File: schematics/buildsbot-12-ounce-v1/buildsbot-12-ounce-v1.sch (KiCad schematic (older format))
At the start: 15 parts

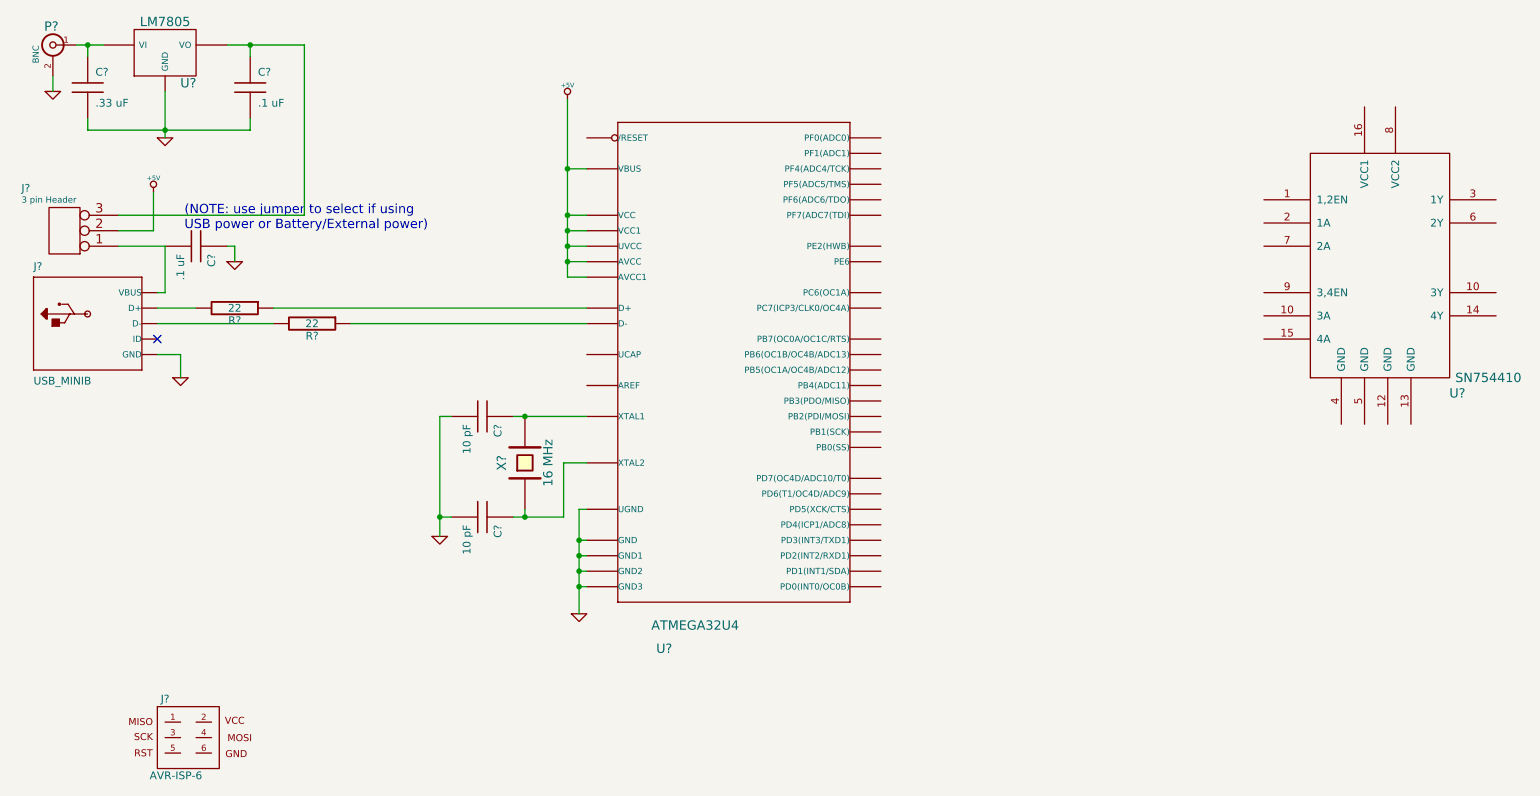
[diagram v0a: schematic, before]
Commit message: Continued working on schematic
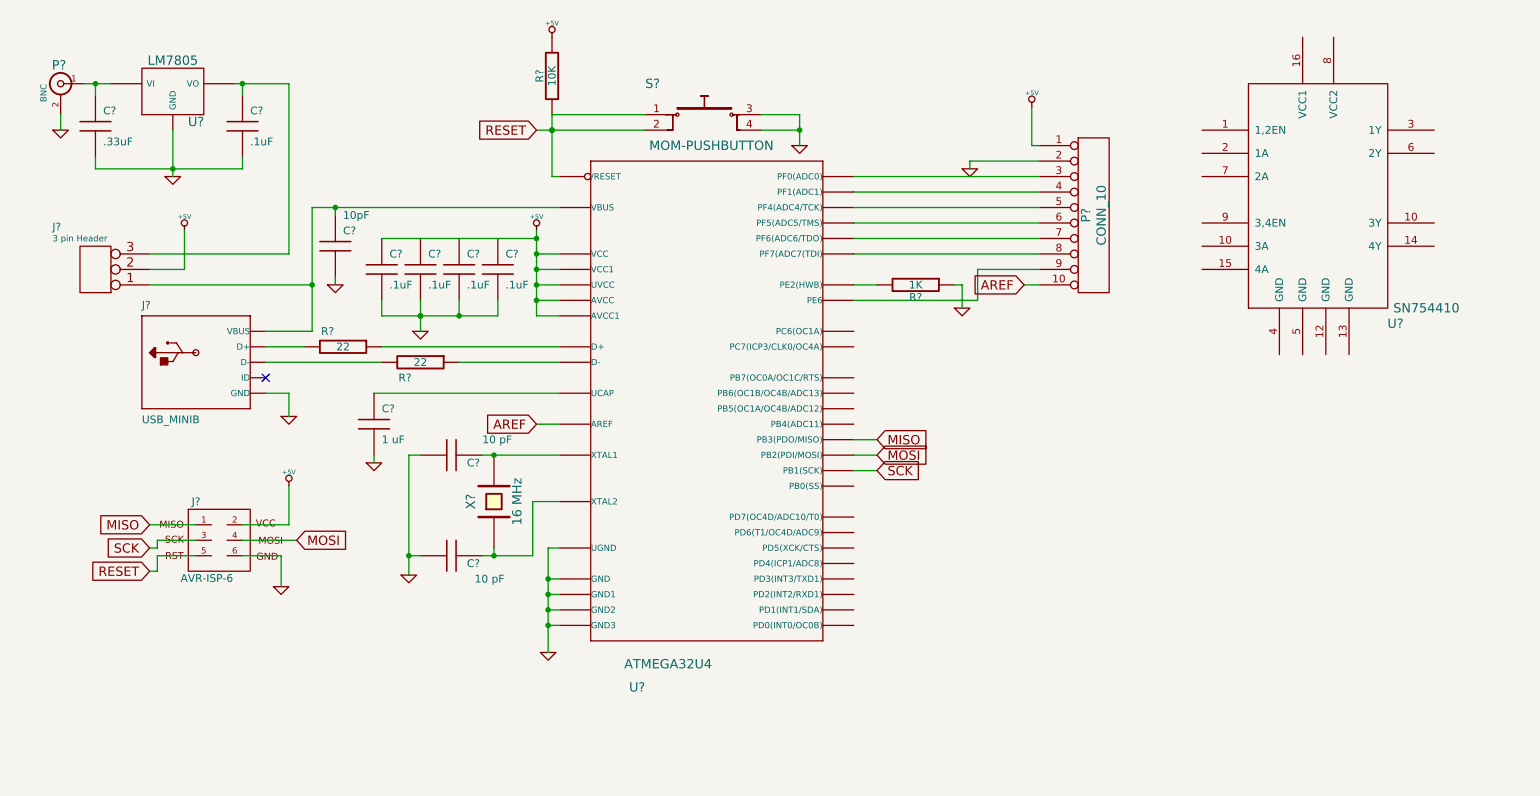
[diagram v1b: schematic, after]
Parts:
- added C?: 1 uF, symbol C
- added C? (x4): .1uF, symbol C
- added P?: CONN_10, symbol CONN_10
- added R?: 10K, symbol R
- added R?: 1K, symbol R
- added S?: MOM-PUSHBUTTON, symbol MOM-PUSHBUTTON
- C?: value .33 uF -> .33uF
- C?: value .1 uF -> .1uF
- C?: value .1 uF -> 10pF
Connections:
- net +5V: now also J?.2, C?.1, P?.1 (P1), R?.2; no longer U?.7 (VBUS)
- net GND: now also C?.2, J?.6, C?.2, C?.2, C?.2, C?.2, C?.2, P?.2 (P2), R?.1, S?.3, S?.4; no longer C?.1
- net MISO: now reaches J?.1
- net MISO: now also U?.11 (PB3(PDO/MISO))
- net SCK: now reaches J?.3
- net SCK: now also U?.9 (PB1(SCK))
- net MOSI: now reaches J?.4
- net MOSI: now also U?.10 (PB2(PDI/MOSI))
- net RESET: now reaches J?.5
- net RESET: now also U?.13 (/RESET), R?.1, S?.1, S?.2
- net at J?.1 (P1), J?.VBUS: now also C?.1, U?.7 (VBUS); no longer C?.2
- net at U?.1 (PE6): now also P?.9 (P9)
- net at U?.33 (PE2(HWB)): now also R?.2
- net at U?.36 (PF7(ADC7(TDI)): now also P?.8 (P8)
- net at U?.37 (PF6(ADC6/TDO)): now also P?.7 (P7)
- net at U?.38 (PF5(ADC5/TMS)): now also P?.6 (P6)
- net at U?.39 (PF4(ADC4/TCK)): now also P?.5 (P5)
- net at U?.40 (PF1(ADC1)): now also P?.4 (P4)
- net at U?.41 (PF0(ADC0)): now also P?.3 (P3)
- net AREF: now reaches U?.42 (AREF)
- net AREF: now also P?.10 (P10)
- net at U?.6 (UCAP): now also C?.1
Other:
- note removed: "(NOTE: use jumper to select if using \nUSB power or Battery/External power)\n"
- moved on the sheet: C?, J?, P?, R?, U?, X?
